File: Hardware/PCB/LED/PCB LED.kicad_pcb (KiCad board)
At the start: 2 copper layers, 22 x 10.5 mm, 7 parts, among them J1 Conn_01x04

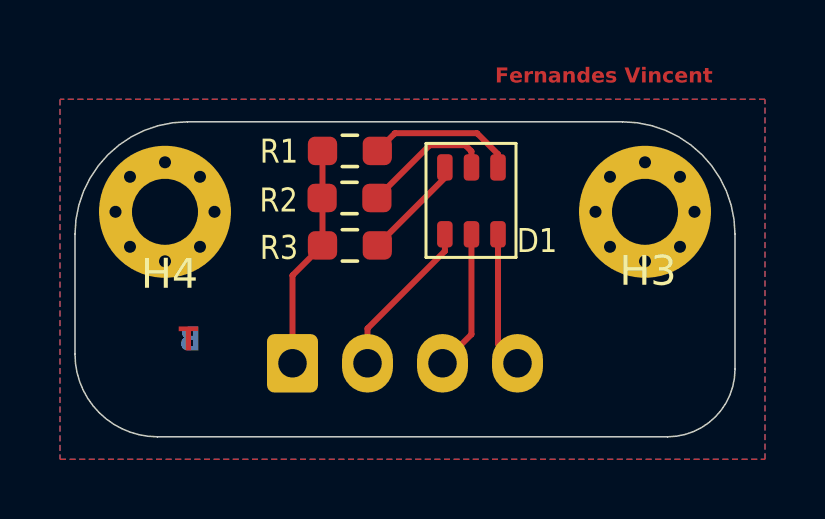
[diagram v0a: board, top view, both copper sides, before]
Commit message: update eye
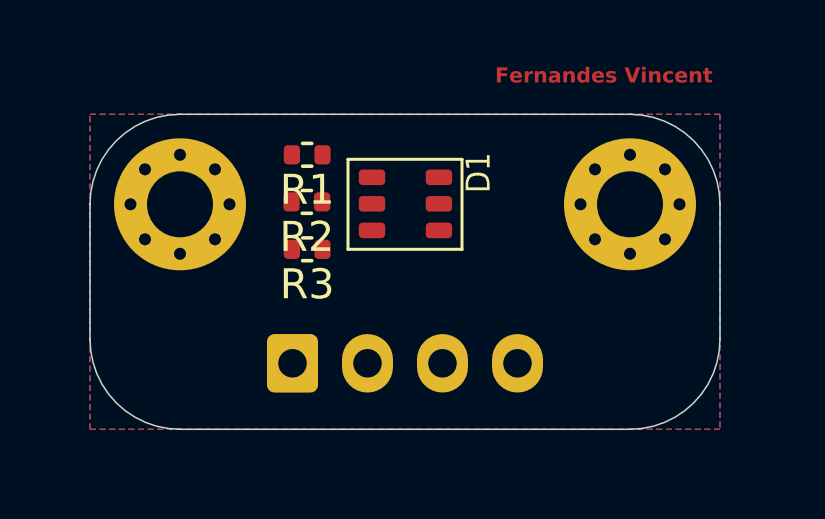
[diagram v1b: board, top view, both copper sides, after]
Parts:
- R1, R2, R3: footprint Resistor_SMD:R_0603_1608Metric_Pad0.98x0.95mm_HandSolder -> Resistor_SMD:R_0402_1005Metric
- moved D1 3.34 mm to (52.5, 88.0), turned to 0 degrees
- moved R1 1.43 mm to (49.2, 86.3)
- moved R2 1.43 mm to (49.2, 87.9)
- moved R3 1.43 mm to (49.2, 89.5)
- moved H3 0.56 mm to (60.0, 88.0)
- moved H4 0.56 mm to (45.0, 88.0)
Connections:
- H3 pad 1: GND -> +5V
- H4 pad 1: GND -> +5V
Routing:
- net +5V: track 7.50 -> 0.00 mm
- net Net-(D1-BK): track 5.37 -> 0.00 mm
- net Net-(D1-RA): track 5.00 -> 0.00 mm
- net Net-(D1-GK): track 4.70 -> 0.00 mm
- net Net-(D1-RK): track 4.57 -> 0.00 mm
- net Net-(D1-GA): track 4.50 -> 0.00 mm
- net Net-(D1-BA): track 3.53 -> 0.00 mm
- added copper zone on B.Cu, net +5V
- added copper zone on F.Cu, net +5V
- removed copper zone on B.Cu, net GND
- removed copper zone on F.Cu, net GND
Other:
- board size 22 x 10.5 mm -> 21 x 10.5 mm
- board text removed: "B"
- board text removed: "T"
